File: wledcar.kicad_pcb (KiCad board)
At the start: 2 copper layers, 41.6 x 46.2 mm, 35 parts, among them J1 Conn_01x04, J2 USB_C_Receptacle_USB2.0_16P, J3 Screw_Terminal_01x02, J8 Screw_Terminal_01x08, U1 SN74AHCT125N, U2 XL4015, U3 AMS1117-3.3, U4 ESP32-S3-WROOM-1

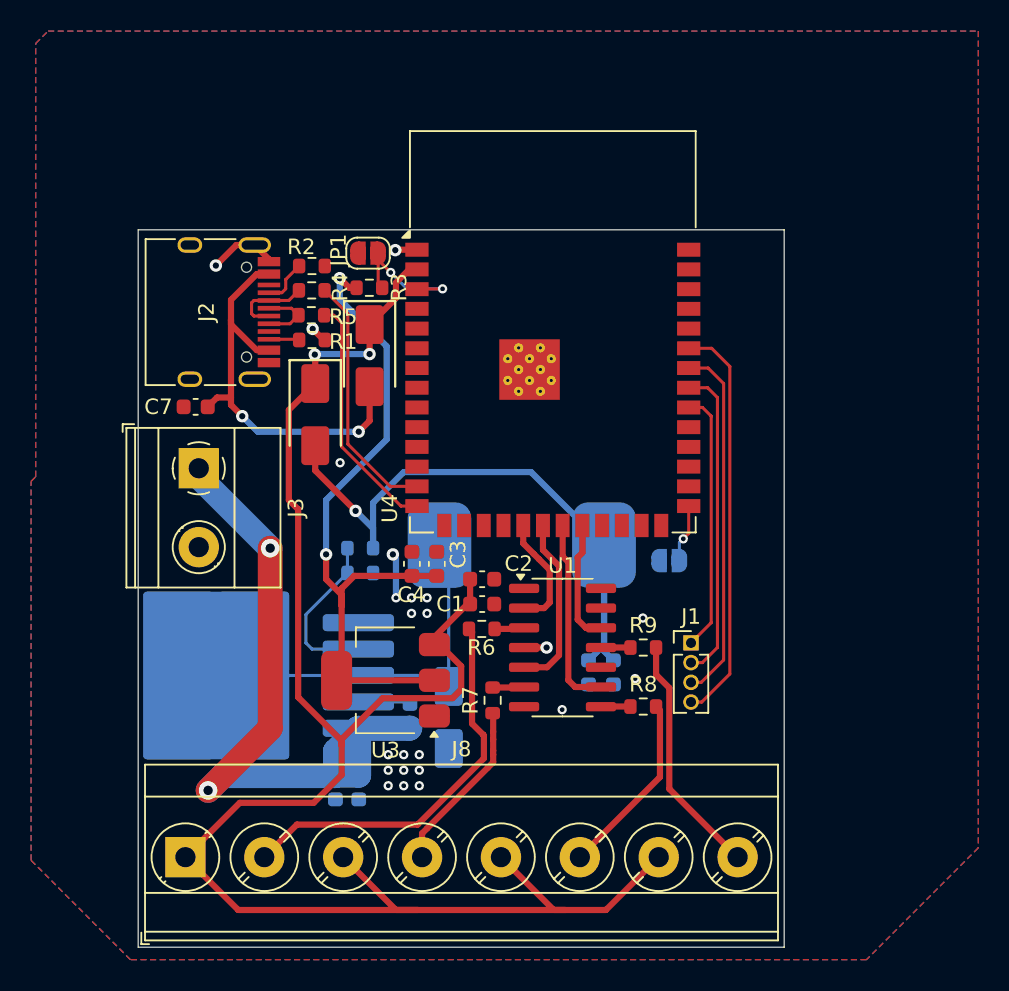
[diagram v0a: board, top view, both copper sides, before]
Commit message: redid the whole pcb 	modified:   wledcar.kicad_pcb 	modified:   wledcar.kicad_pro 	modified:   wledcar.kicad_sch
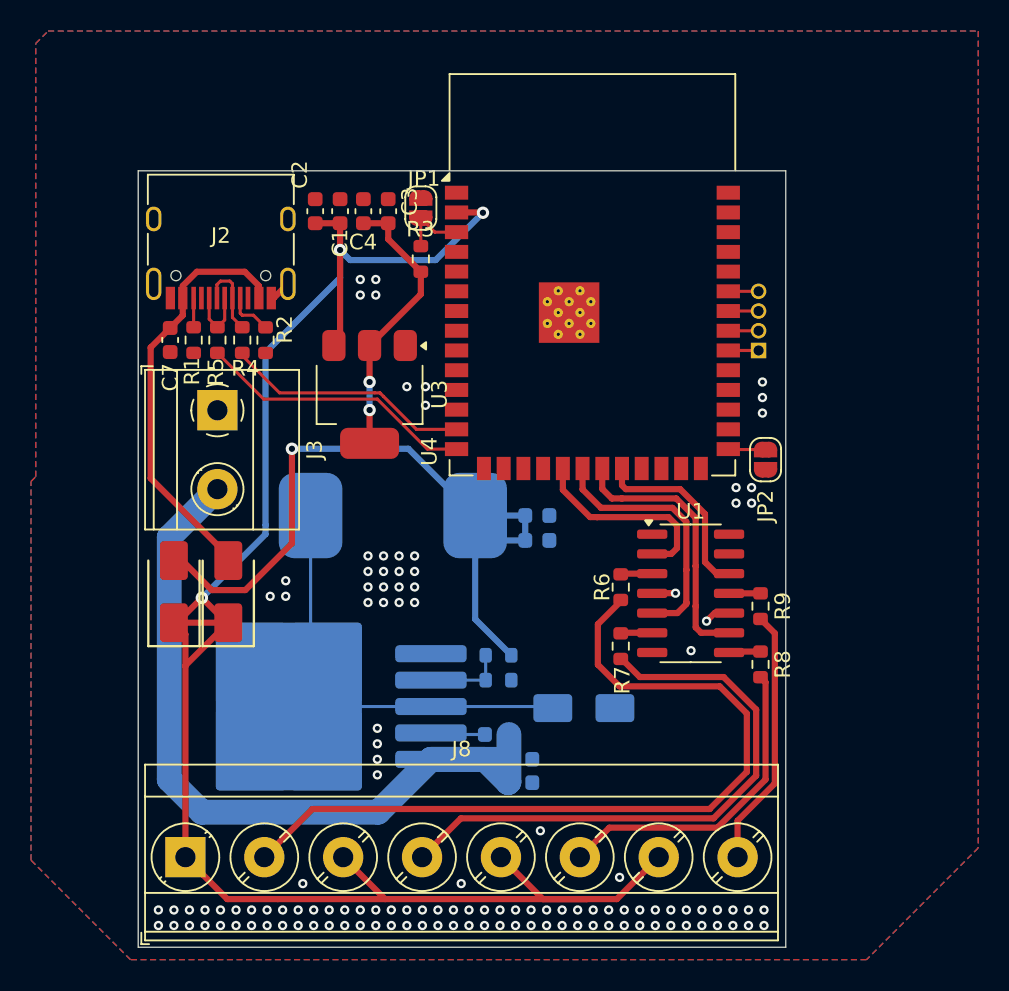
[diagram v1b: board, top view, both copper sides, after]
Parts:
- J1: moved to B.Cu
- JP2: moved to F.Cu
- moved C1 26.9 mm to (211.6, 92.7), turned to 90 degrees
- moved C2 26.0 mm to (210.0, 92.7), turned to 90 degrees
- moved C3 22.9 mm to (214.7, 92.7)
- moved C4 22.9 mm to (213.1, 92.7)
- moved J1 19.3 mm to (238.6, 101.7)
- moved U3 18.4 mm to (213.5, 104.5), turned to -90 degrees
- moved D3 17.7 mm to (204.4, 117.2), turned to 90 degrees
- moved D1 14.6 mm to (200.9, 117.2), turned to 90 degrees
- moved C8 11.9 mm to (223.2, 129.5), turned to 180 degrees
- moved R10 11.3 mm to (221.8, 122.9)
- moved R11 11.3 mm to (221.8, 121.3)
- moved C9 11.2 mm to (224.3, 112.3), turned to 180 degrees
- moved C11 10.6 mm to (223.2, 128.0), turned to 180 degrees
- moved R6 9.35 mm to (229.7, 116.9), turned to 90 degrees
- moved C12 9.12 mm to (224.3, 113.9), turned to 180 degrees
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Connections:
- J3 pad 1: +12V -> GND
- J3 pad 2: GND -> +12V
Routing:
- net LED1: track 25.5 -> 52.7 mm
- net LED2: track 11.2 -> 38.0 mm
- net VDD: track 44.5 -> 18.0 mm
- net Net-(J1-Pin_4): track 26.2 -> 1.95 mm
- net Net-(J1-Pin_3): track 23.2 -> 1.95 mm
- net Net-(J1-Pin_2): track 20.3 -> 1.95 mm
- net Net-(J1-Pin_1): track 16.8 -> 1.95 mm
- net LED3: track 11.9 -> 20.8 mm
- net +12V: track 44.4 -> 52.8 mm, vias 2 -> 0
- net GND: track 12.1 -> 4.62 mm, vias 23 -> 124
- net Net-(U2-FB): track 10.7 -> 5.13 mm
- net MCULED1: track 7.46 -> 12.9 mm
- net MCULED2: track 11.4 -> 16.6 mm
- net MCULED3: track 12.4 -> 17.4 mm
- net Net-(JP1-B): track 9.36 -> 4.47 mm, vias 2 -> 0
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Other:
- board size 41.6 x 46.2 mm -> 41.7 x 50 mm
